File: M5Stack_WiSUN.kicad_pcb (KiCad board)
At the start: 2 copper layers, 50 x 50 mm, 23 parts, among them J1 MBUS_TOP, J2 MBUS_BOTTOM, J3 AVR_IO, J4 ISP, U1 BP35A1, U2 ATMEGA328P-AU

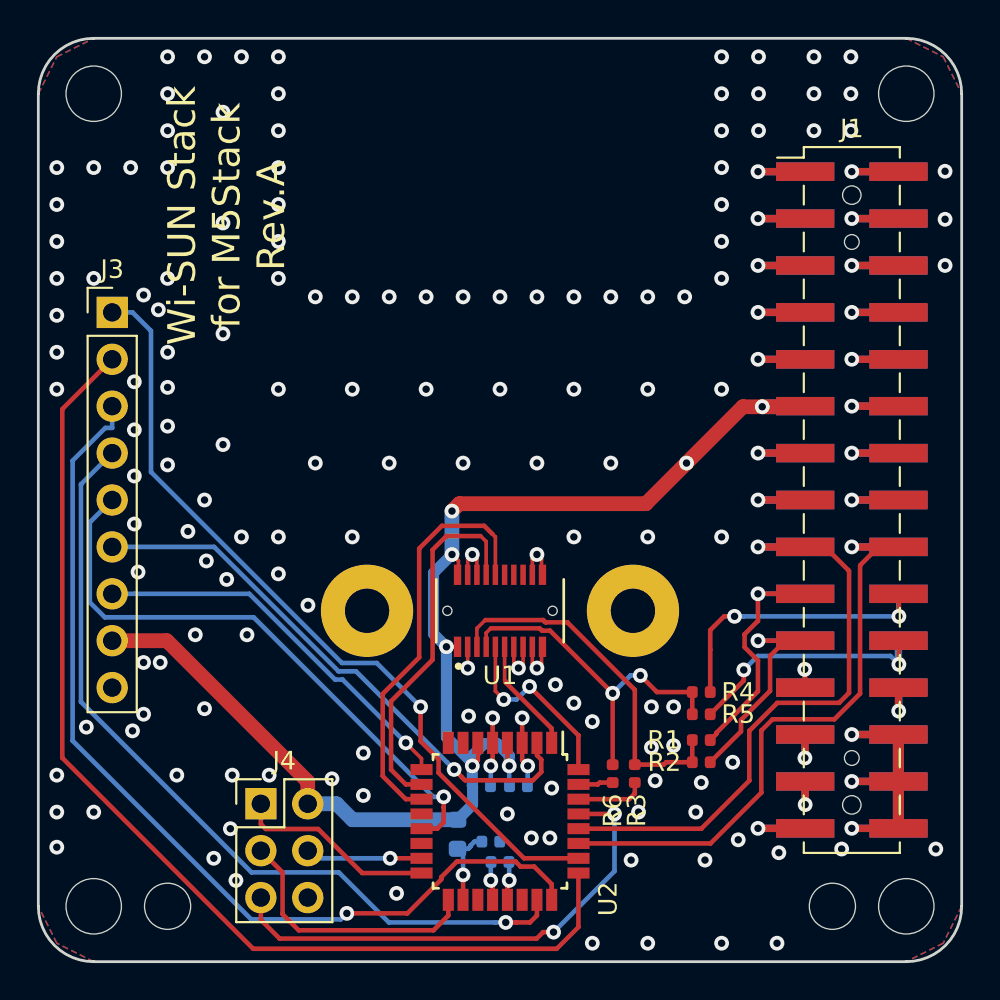
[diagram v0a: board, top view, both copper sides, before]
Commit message: PCB revision B
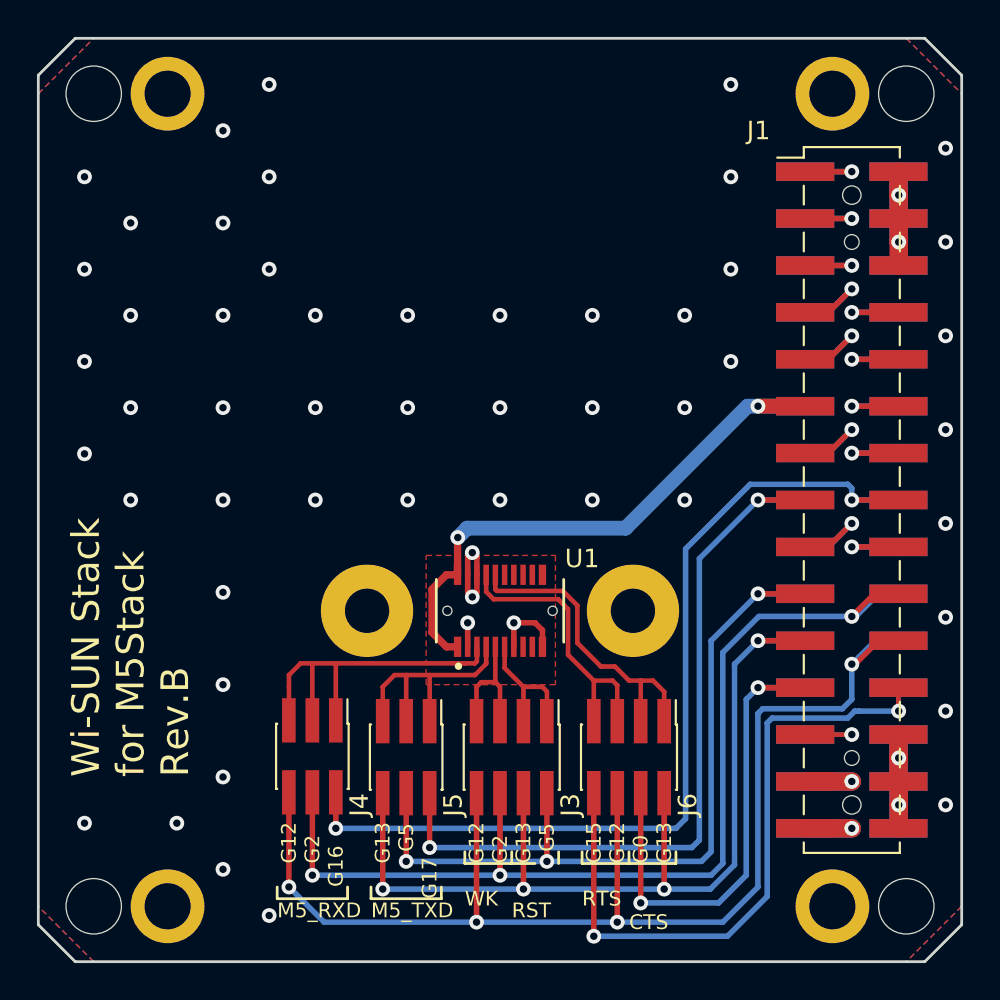
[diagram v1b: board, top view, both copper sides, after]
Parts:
- removed C1, C2, C3, C4: 100n, Capacitor_SMD:C_0402_1005Metric
- removed L1: 10u, Inductor_SMD:L_0603_1608Metric
- removed R1, R4: 0, Resistor_SMD:R_0402_1005Metric
- removed R2, R3, R5, R6: NMT, Resistor_SMD:R_0402_1005Metric
- removed U2: ATMEGA328P-AU, Package_QFP:LQFP-32_7x7mm_P0.8mm
- added J5: PH127-2x3MG, Connector_PinHeader_1.27mm:PinHeader_2x03_P1.27mm_Vertical_SMD, F.Cu at (29.9, 78.9)
- added J6: PH127-2x4MG, Connector_PinHeader_1.27mm:PinHeader_2x04_P1.27mm_Vertical_SMD, F.Cu at (42.0, 78.9)
- added MH7: Fix, MountingHole:MountingHole_2.5mm_Pad, F.Cu at (17.0, 43.0)
- added MH8: Fix, MountingHole:MountingHole_2.5mm_Pad, F.Cu at (53.0, 43.0)
- J3: value AVR_IO -> PH127-2x4MG; footprint Connector_PinHeader_2.54mm:PinHeader_1x09_P2.54mm_Vertical -> Connector_PinHeader_1.27mm:PinHeader_2x04_P1.27mm_Vertical_SMD
- J4: value ISP -> PH127-2x3MG; footprint Connector_PinHeader_2.54mm:PinHeader_2x03_P2.54mm_Vertical -> Connector_PinHeader_1.27mm:PinHeader_2x03_P1.27mm_Vertical_SMD
- MH5, MH6: footprint MountingHole:MountingHole_2.5mm -> MountingHole:MountingHole_2.5mm_Pad
- moved J3 32.4 mm to (35.6, 78.9), turned to 270 degrees
- moved J4 3.79 mm to (24.8, 78.9), turned to 270 degrees
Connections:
- J3 pad 1: /AVR_ADC3 -> /BP35_RESET
- J3 pad 2: /AVR_ADC2 -> /GPIO_G5
- J3 pad 3: /AVR_ADC1 -> /BP35_RESET
- J3 pad 4: /AVR_ADC0 -> /IIS_WS
- J3 pad 5: /AVR_PB1 -> /BP35_WKUP
- J3 pad 6: /AVR_PD4 -> /GPIO_G2
- J3 pad 7: /AVR_PD5 -> /BP35_WKUP
- J3 pad 8: +3V3 -> /IIS_SK
- J4 pad 1: /AVR_MISO -> /BP35_TXD
- J4 pad 2: +3V3 -> /RXD2
- J4 pad 3: /AVR_SCK -> /BP35_TXD
- J4 pad 4: /AVR_MOSI -> /GPIO_G2
- J4 pad 5: /AVR_RESET -> /BP35_TXD
- J4 pad 6: GND -> /IIS_SK
- U1 pad 16: (no net) -> Net-(U1-Pad16)
- U1 pad 17: (no net) -> Net-(U1-Pad17)
- U1 pad 18: (no net) -> Net-(U1-Pad18)
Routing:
- net /AVR_ADC2: track 58.3 -> 0.00 mm
- net /IIS_SK: track 14.6 -> 68.9 mm, vias 2 -> 4
- net /AVR_ADC1: track 51.9 -> 0.00 mm, vias 1 -> 0
- net /RXD2: track 5.07 -> 51.9 mm, vias 1 -> 2
- net /AVR_ADC0: track 44.8 -> 0.00 mm, vias 1 -> 0
- net /AVR_ADC3: track 43.5 -> 0.00 mm, vias 1 -> 0
- net +3V3: track 74.9 -> 32.1 mm, vias 7 -> 2
- net /GPIO_G2: track 16.3 -> 56.7 mm, vias 2 -> 3
- net /IIS_WS: track 14.5 -> 53.0 mm, vias 1 -> 4
- net /TXD2: track 5.13 -> 42.6 mm, vias 1 -> 2
- net /IIS_OUT: track 2.55 -> 37.4 mm, vias 1 -> 2
- net /AVR_PB1: track 32.3 -> 0.00 mm, vias 1 -> 0
- net /AVR_PD4: track 30.3 -> 0.00 mm, vias 1 -> 0
- net /SDA: track 35.1 -> 5.05 mm
- net /GPIO_G5: track 15.8 -> 44.2 mm, vias 1 -> 3
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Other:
- outline, holes or cut-outs redrawn
- board text added: "CTS"
- board text added: "G0"
- board text added: "G12"
- board text added: "G13"
- board text added: "G15"
- board text added: "G16"
- board text added: "G17"
- board text added: "G2"
- board text added: "G5"
- board text added: "M5_RXD"
- board text added: "M5_TXD"
- board text added: "RST"
- board text added: "RTS"
- board text added: "WK"
- board text added: "Wi-SUN Stack for M5Stack Rev.B"
- board text removed: "Wi-SUN Stack for M5Stack Rev.A"
